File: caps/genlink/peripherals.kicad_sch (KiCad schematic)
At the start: 36 parts, among them J11 UEXT, J12 SM04B-SRSS-TB, J8 XKTF-0803-0, J9 U254-051T-4BH81-S2S, Q1 BSS138, SW3 PROG_EN, U3 CH340C, U4 PCF8563T, Y1 32kHz

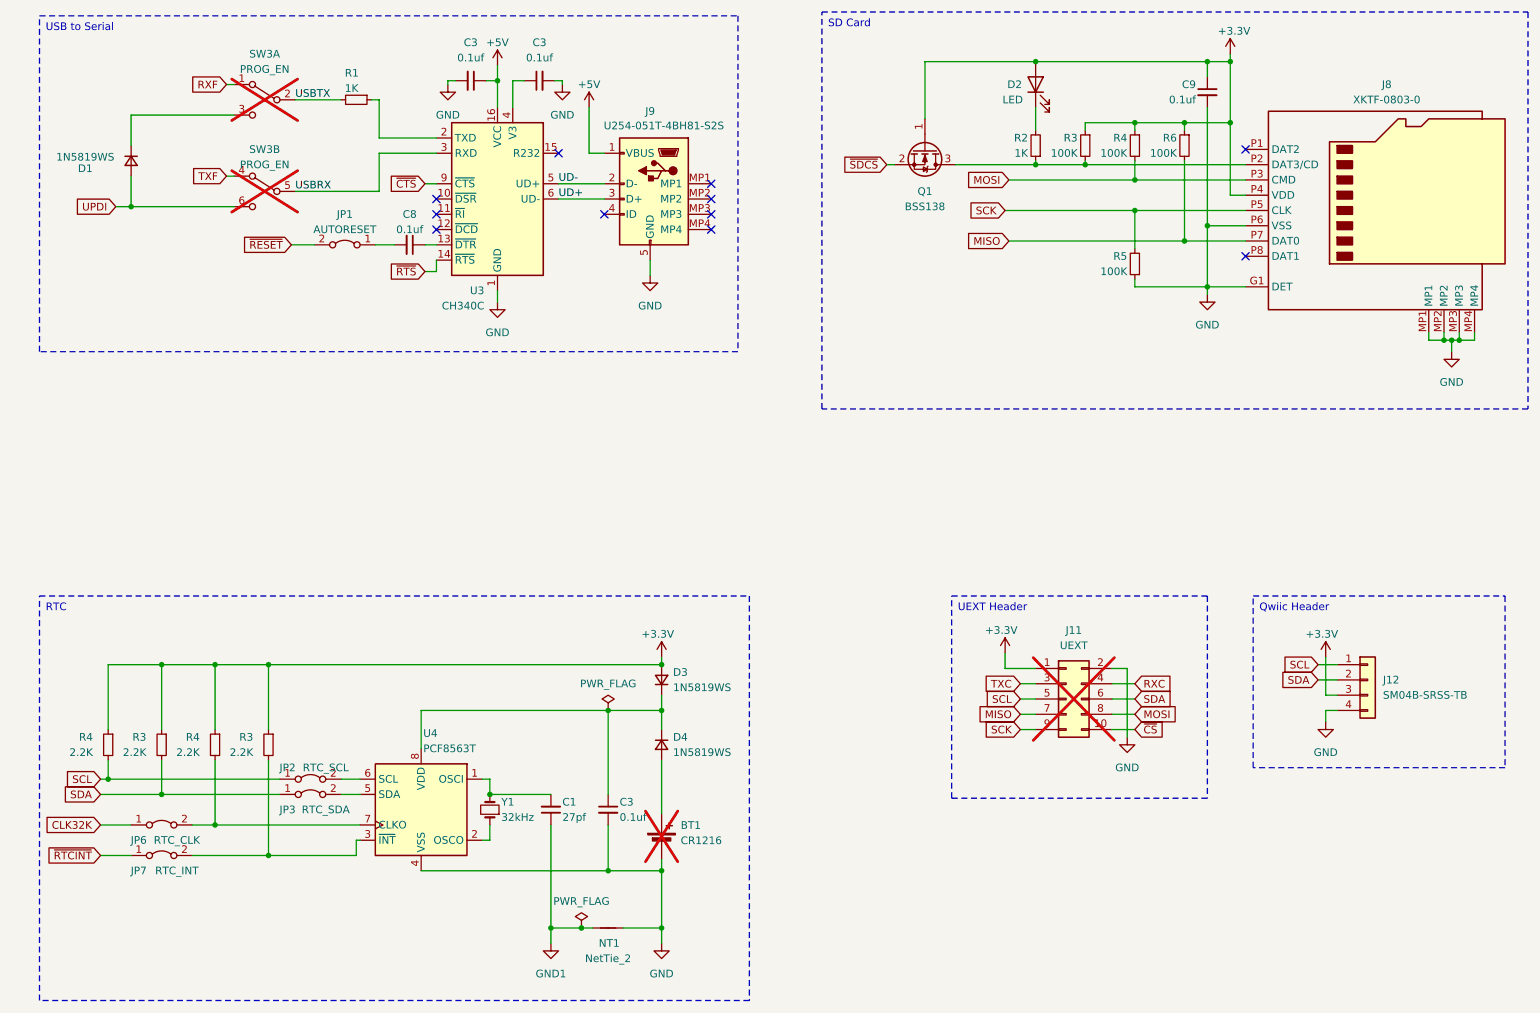
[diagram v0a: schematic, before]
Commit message: Add LCSC part numbers
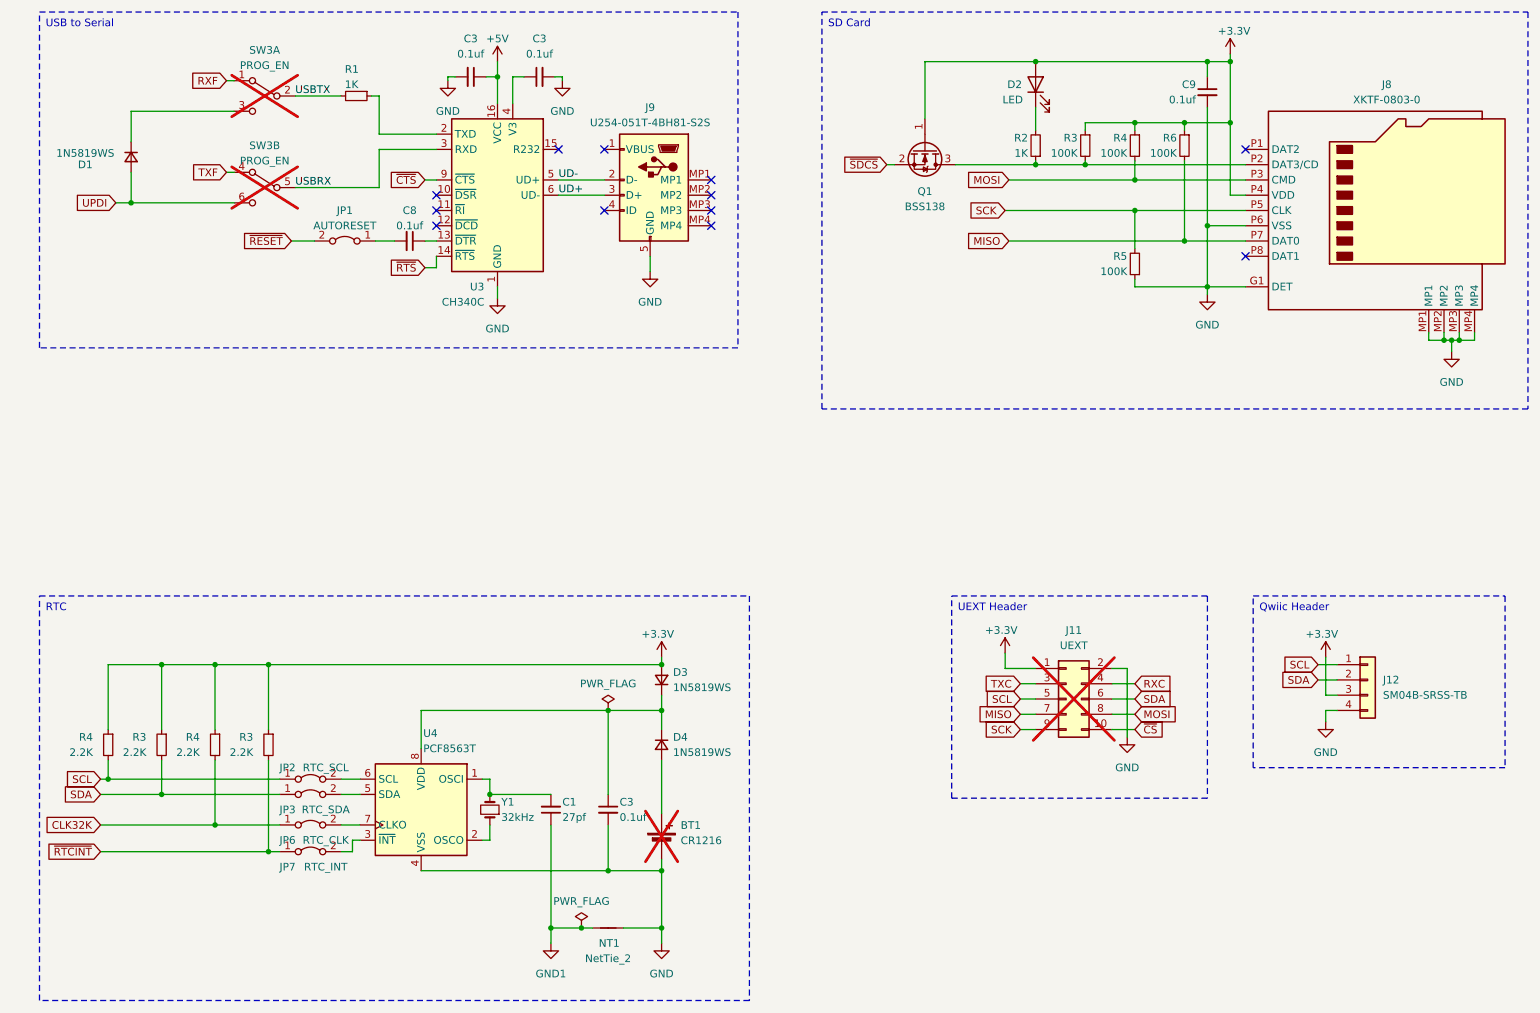
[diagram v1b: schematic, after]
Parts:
- C1: LCSC part number C107045 -> (none)
- C3, C8, C9: LCSC part number C1525 -> (none)
- D1, D3, D4: LCSC part number C64886 -> (none)
- D2: footprint LED_SMD:LED_0603_1608Metric -> LED_SMD:LED_0805_2012Metric; LCSC part number C2286 -> (none)
- J12: footprint SamacSys_Parts:SM04B-SRSS-TB_LFSN_ -> Custom:JST_SM04B-SRSS-TB_LF__SN_; LCSC part number C160404 -> (none)
- J8: LCSC part number C381083 -> (none)
- J9: LCSC part number C381144 -> (none)
- JP6, JP7: footprint Jumper:SolderJumper-2_P1.3mm_Open_RoundedPad1.0x1.5mm -> Jumper:SolderJumper-2_P1.3mm_Bridged_RoundedPad1.0x1.5mm
- Q1: LCSC part number C7420339 -> (none)
- R1, R2: LCSC part number C11702 -> (none)
- R3, R4: LCSC part number C25879 -> (none)
- R3, R4, R5, R6: LCSC part number C25741 -> (none)
- U3: LCSC part number C7464026 -> (none)
- Y1: LCSC part number C32346 -> (none)
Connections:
- net +5V: no longer J9.1 (VBUS)
- net CLK32K: now also R4.2
- net ~{RTCINT}: now also R3.2
- net at JP7.2 (B), U4.3 (~{INT}): no longer R3.2
- net at JP6.2 (B), U4.7 (CLKO): no longer R4.2
- no-connect marks 11 -> 12
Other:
- moved on the sheet: C3, C8, D1, J9, JP1, JP6, JP7, R1, SW3A, SW3B, U3
